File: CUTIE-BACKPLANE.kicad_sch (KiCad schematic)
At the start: 0 parts

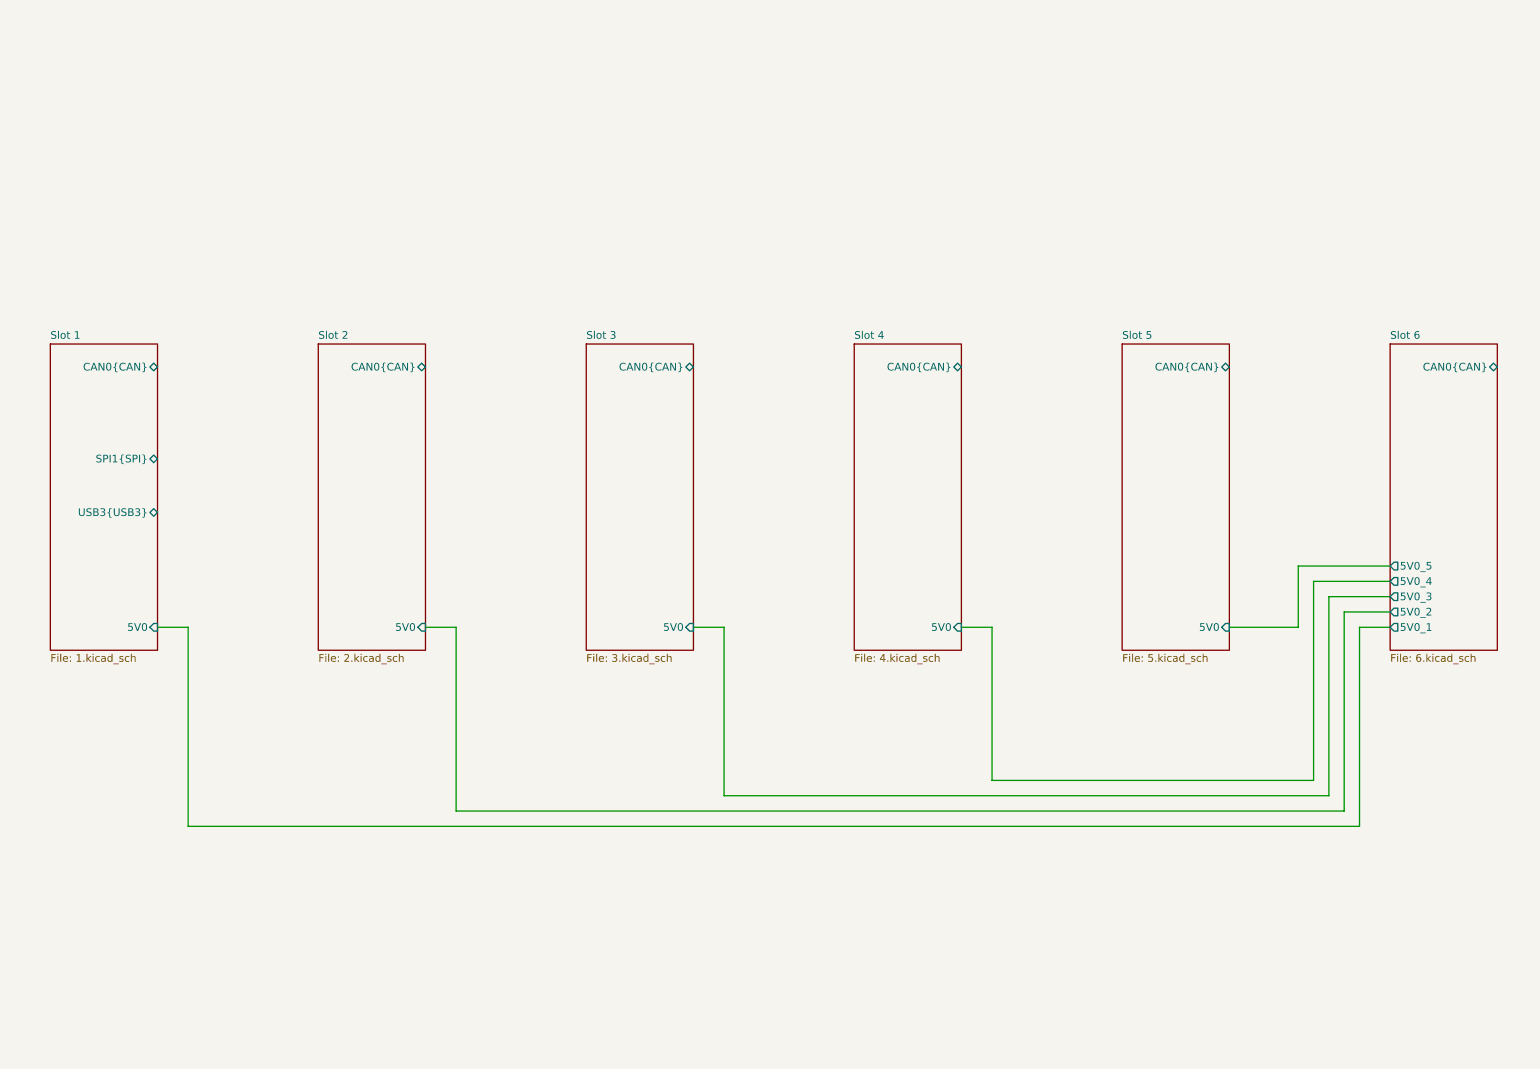
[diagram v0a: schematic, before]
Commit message: final setup for power rails
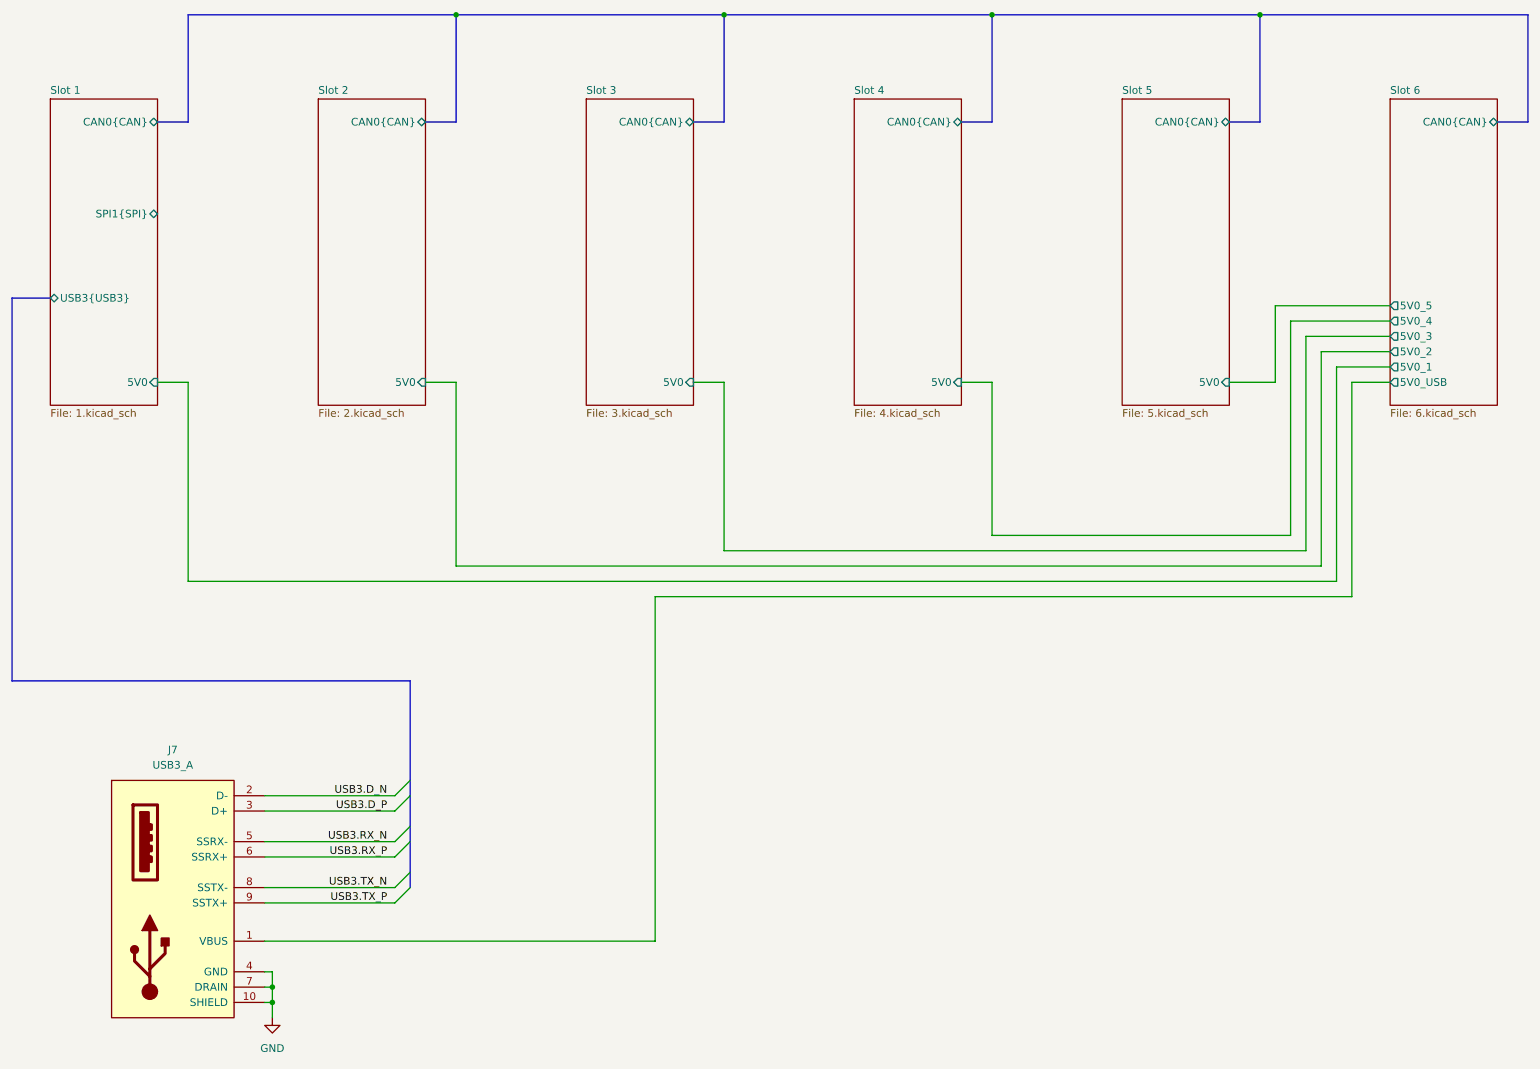
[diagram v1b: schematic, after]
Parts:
- added J7: USB3_A, symbol Connector:USB3_A
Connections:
- new net GND: J7.10 (SHIELD), J7.4 (GND), J7.7 (DRAIN)
- new net Slot 6/5V0_USB: J7.1 (VBUS)
- new net USB3.D_N: J7.2 (D-)
- new net USB3.D_P: J7.3 (D+)
- new net USB3.RX_N: J7.5 (SSRX-)
- new net USB3.RX_P: J7.6 (SSRX+)
- new net USB3.TX_N: J7.8 (SSTX-)
- new net USB3.TX_P: J7.9 (SSTX+)
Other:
- sheet Slot 6 ports: added 5V0_USB; removed none

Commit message: initialized for 4-card
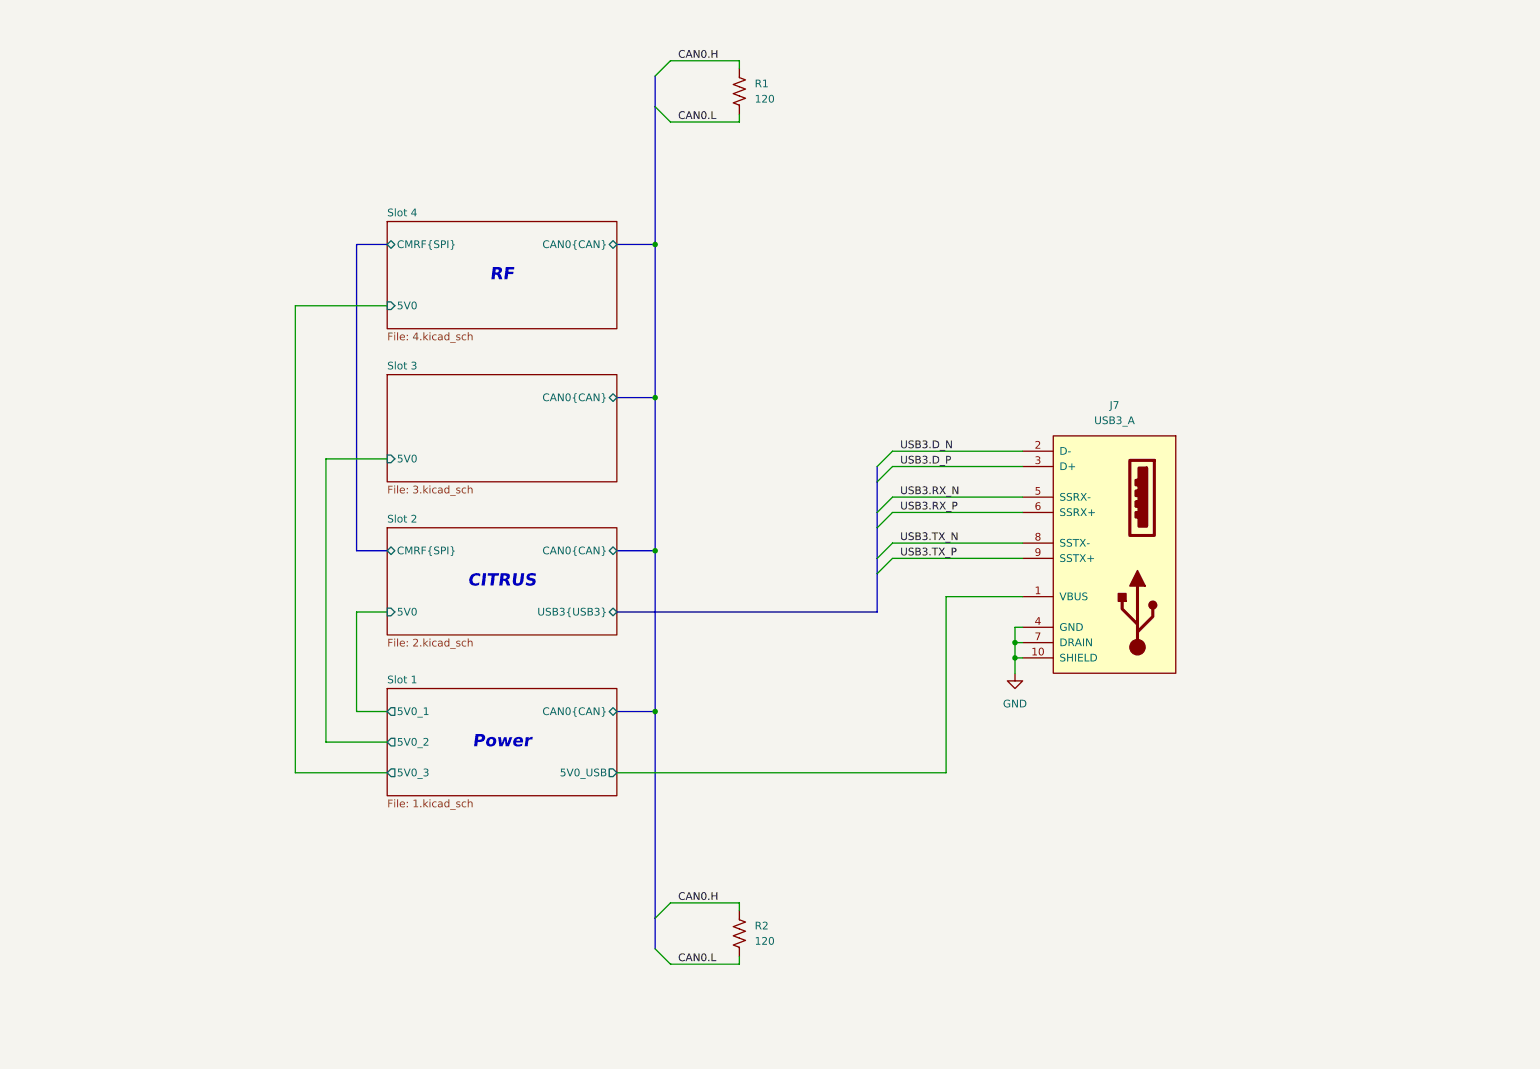
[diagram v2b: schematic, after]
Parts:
- added R1, R2: 120, Resistor_SMD:R_0603_1608Metric, symbol Device:R_US
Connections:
- net Slot 6/5V0_USB renamed Slot 1/5V0_USB
- new net CAN0.H: R1.1, R2.1
- new net CAN0.L: R1.2, R2.2
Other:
- removed sheet Slot 5
- removed sheet Slot 6
- sheet Slot 1 ports: added 5V0_1, 5V0_2, 5V0_3, 5V0_USB; removed 5V0, SPI1{SPI}, USB3{USB3}
- sheet Slot 2 ports: added CMRF{SPI}, USB3{USB3}; removed none
- sheet Slot 4 ports: added CMRF{SPI}; removed none
- note added: "CITRUS"
- note added: "Power"
- note added: "RF"
- moved on the sheet: J7
